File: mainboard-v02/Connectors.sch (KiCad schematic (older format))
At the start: 13 parts, among them J1 503182-1852, J2 Conn_01x05, J3 10118194-0001LF, J4 DCJ0303, U8 MR25H40MDF

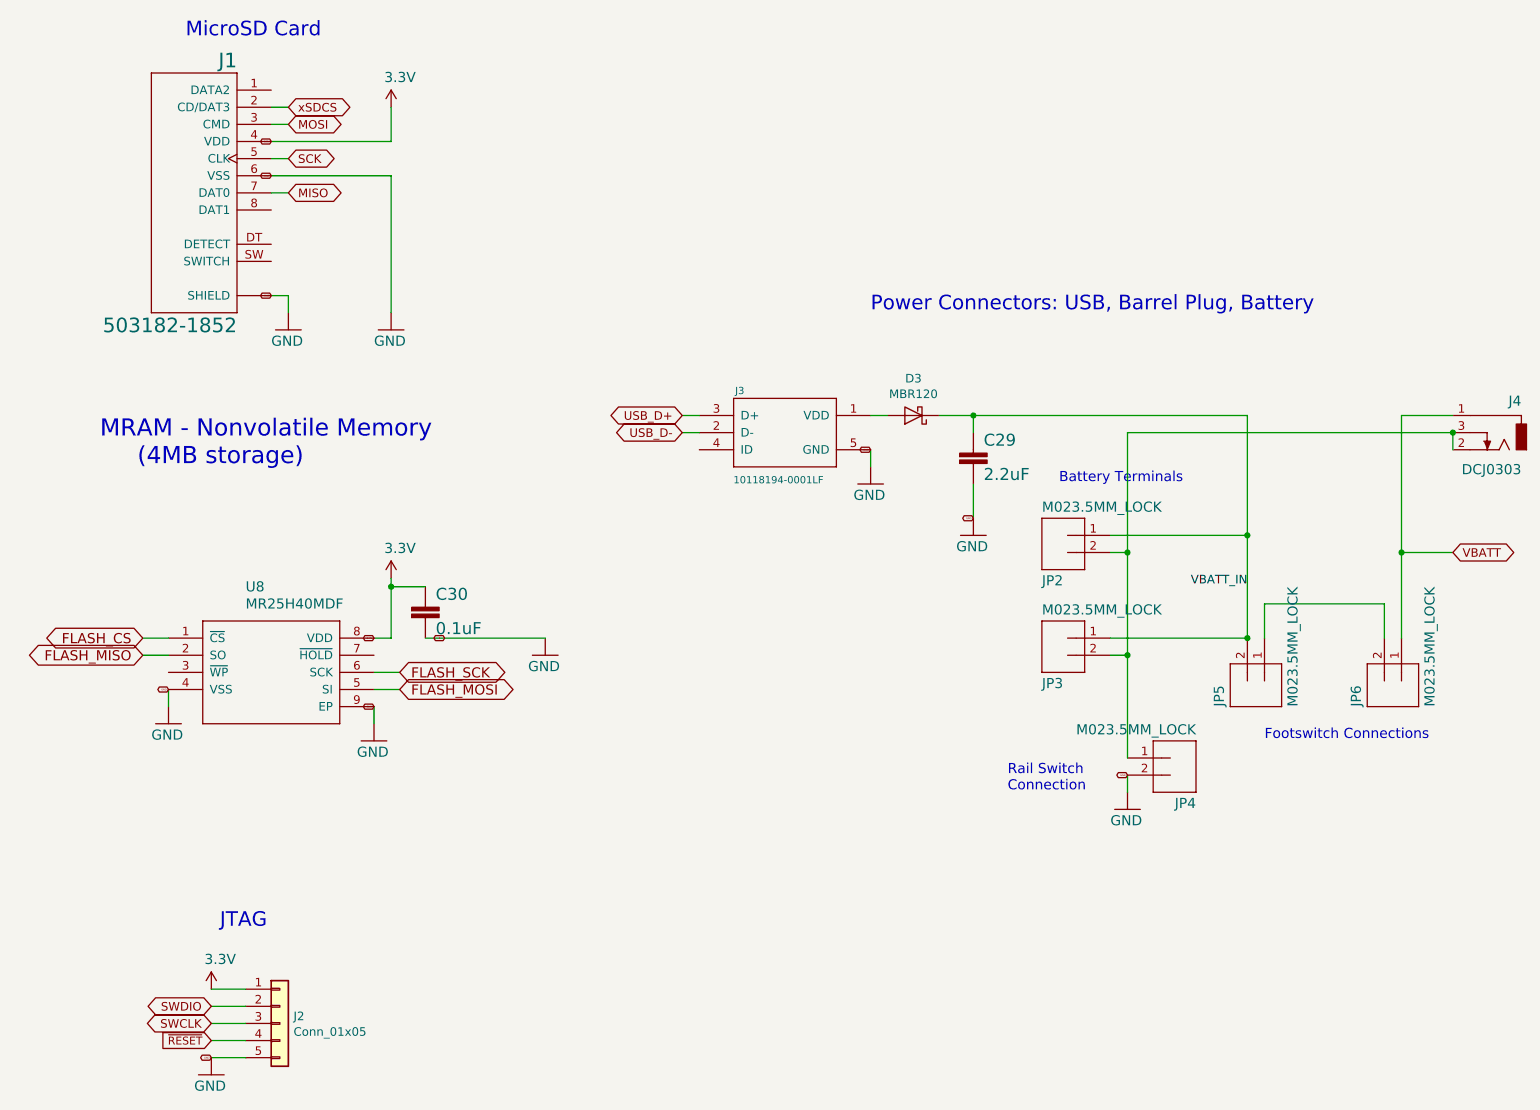
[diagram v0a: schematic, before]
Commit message: fixing bold font and adding schematic pdf of v02
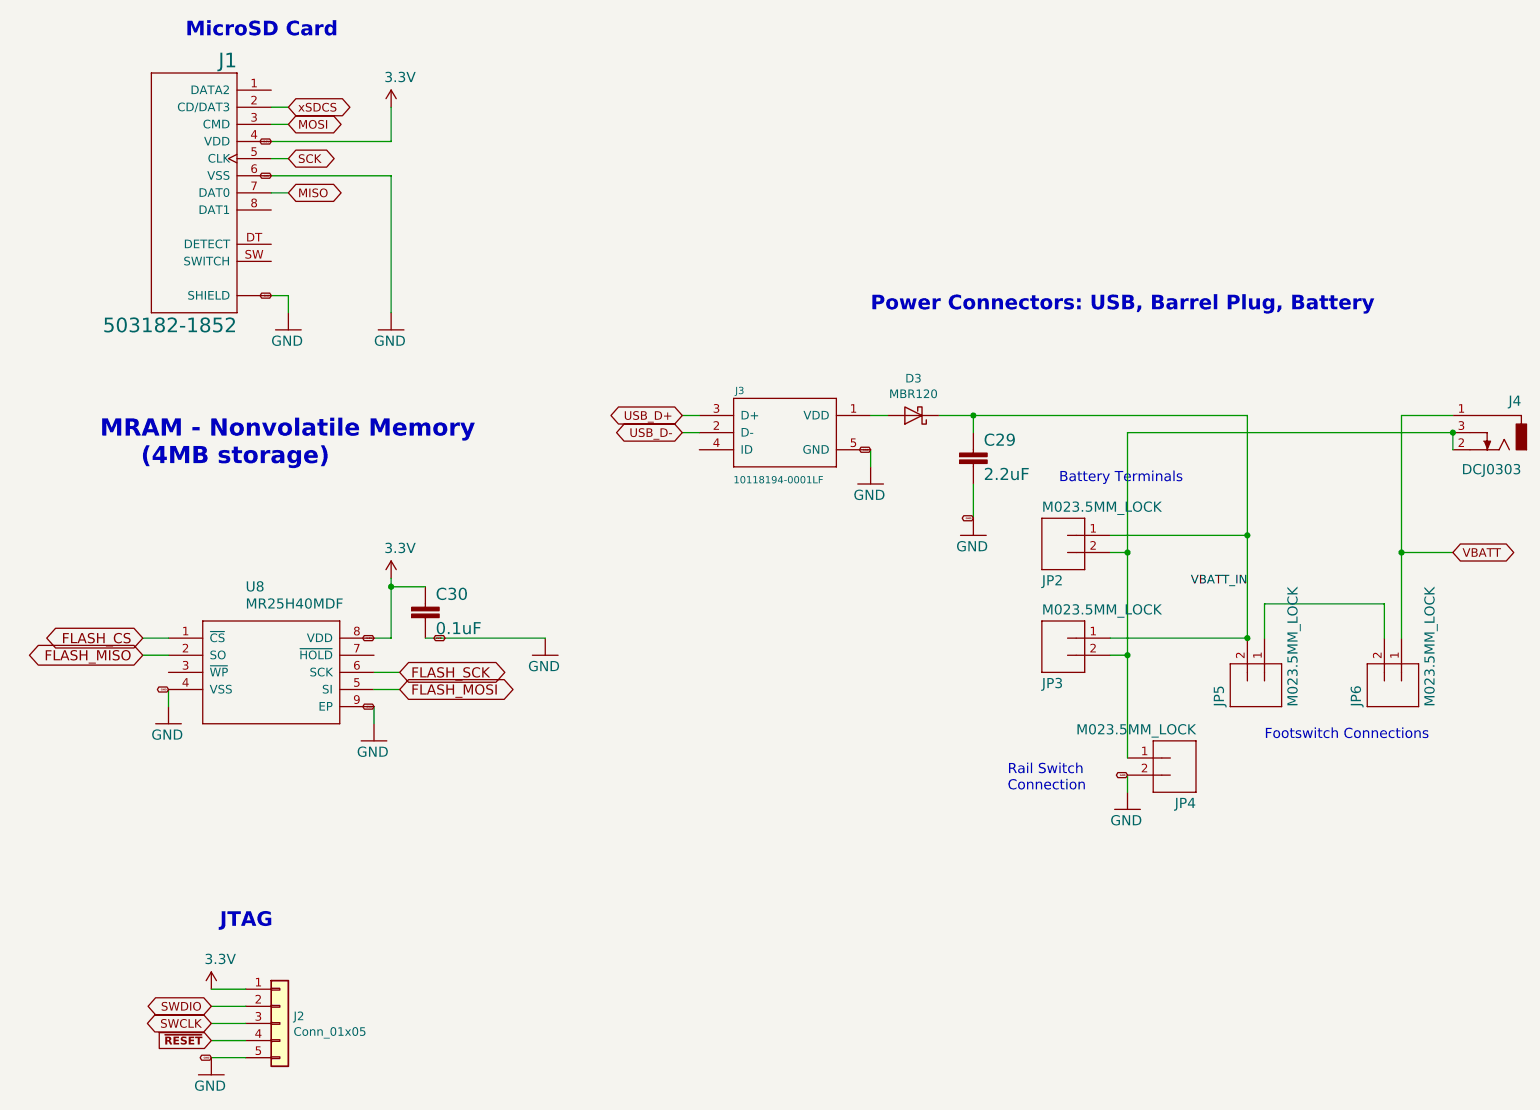
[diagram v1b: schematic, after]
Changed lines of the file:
@@
 EESchema Schematic File Version 4
-LIBS:mainboard
 EELAYER 29 0
 EELAYER END
@@
 Wire Wire Line
 	7900 5200 7900 5300
-Text GLabel 7900 5200 0    10   BiDi ~ 0
+Text GLabel 7900 5200 0    10   BiDi ~ 2
 GND
 Wire Wire Line
 	7000 3700 7000 3500
-Text GLabel 7000 3700 0    10   BiDi ~ 0
+Text GLabel 7000 3700 0    10   BiDi ~ 2
 GND
 Wire Wire Line
 	6400 3300 6400 3400
-Text GLabel 6400 3300 0    10   BiDi ~ 0
+Text GLabel 6400 3300 0    10   BiDi ~ 2
 GND
 Wire Wire Line
@@
 Wire Wire Line
 	3000 2400 3000 2500
-Text GLabel 2900 2400 0    10   BiDi ~ 0
+Text GLabel 2900 2400 0    10   BiDi ~ 2
 GND
 Wire Wire Line
@@
 Wire Wire Line
 	3600 1700 3600 2500
-Text GLabel 2900 1700 0    10   BiDi ~ 0
+Text GLabel 2900 1700 0    10   BiDi ~ 2
 GND
 Wire Wire Line
 	2300 4700 2300 4800
-Text GLabel 2300 4700 0    10   BiDi ~ 0
+Text GLabel 2300 4700 0    10   BiDi ~ 2
 GND
 Wire Wire Line
 	3500 4800 3500 4900
-Text GLabel 3500 4800 0    10   BiDi ~ 0
+Text GLabel 3500 4800 0    10   BiDi ~ 2
 GND
 Wire Wire Line
@@
 Wire Wire Line
 	3600 1500 3600 1300
-Text GLabel 2900 1500 0    10   BiDi ~ 0
+Text GLabel 2900 1500 0    10   BiDi ~ 2
 3.3V
 Wire Wire Line
@@
 Wire Wire Line
 	3600 4400 3600 4100
-Text GLabel 3500 4400 0    10   BiDi ~ 0
+Text GLabel 3500 4400 0    10   BiDi ~ 2
 3.3V
 Text GLabel 2550 6650 0    50   BiDi ~ 0
@@
 Text Notes 7200 5300 0    59   ~ 0
 Rail Switch\nConnection
-Text Notes 2600 6100 0    85   ~ 0
+Text Notes 2600 6100 0    85   ~ 17
 JTAG
-Text Notes 6400 2500 0    85   ~ 0
+Text Notes 6400 2500 0    85   ~ 17
 Power Connectors: USB, Barrel Plug, Battery
-Text Notes 2400 900  0    85   ~ 0
+Text Notes 2400 900  0    85   ~ 17
 MicroSD Card
-Text Notes 1900 3400 0    100  ~ 0
+Text Notes 1900 3400 0    100  ~ 20
 MRAM - Nonvolatile Memory\n     (4MB storage)
 $Comp
@@
 Wire Wire Line
 	2550 6450 2750 6450
-Text GLabel 2550 6850 0    10   BiDi ~ 0
+Text GLabel 2550 6850 0    10   BiDi ~ 2
 GND
 $Comp
@@
 	1    0    0    -1
 $EndComp
-Text GLabel 2550 6750 0    46   Input ~ 0
+Text GLabel 2550 6750 0    46   Input ~ 9
 ~RESET
 Wire Wire Line
@@
 	1    0    0    -1
 $EndComp
-Text GLabel 3850 4400 2    10   BiDi ~ 0
-GND
-$Comp
+Text GLabel 3850 4400 2    10   BiDi ~ 2
+GND
+$Comp
